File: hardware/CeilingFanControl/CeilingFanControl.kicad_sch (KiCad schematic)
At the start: 28 parts, among them J1 Screw_Terminal_01x02, J2 Conn_01x04, J3 Conn_01x04, J4 Screw_Terminal_01x05, Q1 BTA16-600B, Q2 BTA16-600B, Q3 BTA16-600B, U1 4N25, U2 PIC16F628A-IP, U3 MOC3020M, U4 MOC3020M, U5 MOC3020M, Y1 Crystal

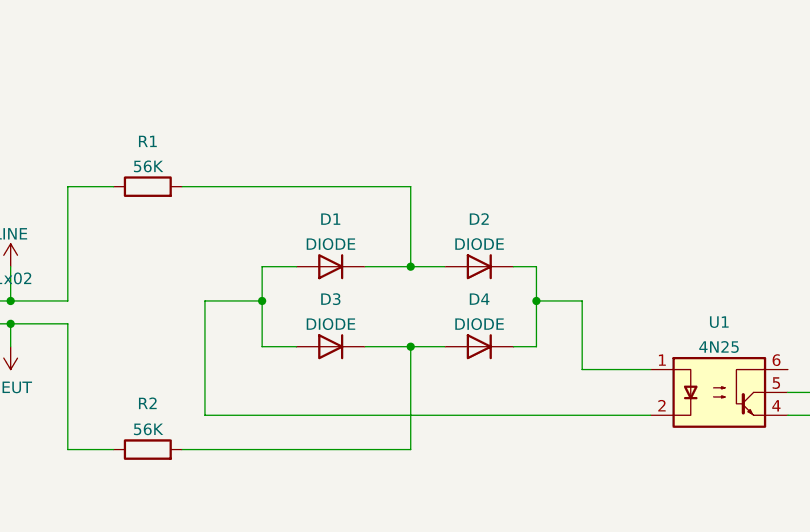
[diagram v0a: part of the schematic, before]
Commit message: Commit befora creating tag
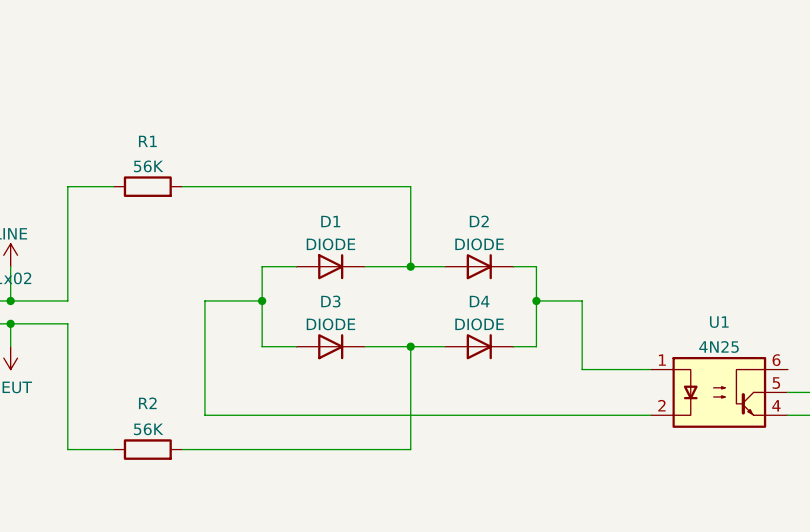
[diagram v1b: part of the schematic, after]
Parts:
- D1, D2, D3, D4: symbol Simulation_SPICE:DIODE -> Diode:1N4001
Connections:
- new net: D2.1 (K), D4.1 (K), U1.1
- new net: D1.1 (K), D2.2 (A), R1.2
- new net: D1.2 (A), D3.2 (A), U1.2
- new net: D3.1 (K), D4.2 (A), R2.2
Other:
- moved on the sheet: D2, D3, D4
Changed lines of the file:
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@@
     (pin "2")
   )
-  (symbol (lib_id "Simulation_SPICE:DIODE") (at 96.52 163.83 0) (mirror x) (unit 1)
-    (in_bom yes) (on_board yes) (fields_autoplaced)
-    (property "Reference" "D2" (id 0) (at 96.52 158.5935 0))
-    (property "Value" "DIODE" (id 1) (at 96.52 161.3686 0))
-    (property "Footprint" "Diode_THT:D_A-405_P7.62mm_Horizontal" (id 2) (at 96.52 163.83 0)
-      (effects (font (size 1.27 1.27)) hide)
-    )
-    (property "Datasheet" "~" (id 3) (at 96.52 163.83 0)
+  (symbol (lib_id "Diode:1N4001") (at 96.52 163.83 180) (unit 1)
+    (in_bom yes) (on_board yes) (fields_autoplaced)
+    (property "Reference" "D2" (id 0) (at 96.52 158.8602 0))
+    (property "Value" "DIODE" (id 1) (at 96.52 161.3971 0))
+    (property "Footprint" "Diode_THT:D_A-405_P7.62mm_Horizontal" (id 2) (at 96.52 159.385 0)
+      (effects (font (size 1.27 1.27)) hide)
+    )
+    (property "Datasheet" "http://www.vishay.com/docs/88503/1n4001.pdf" (id 3) (at 96.52 163.83 0)
       (effects (font (size 1.27 1.27)) hide)
     )
@@
     (pin "1")
   )
-  (symbol (lib_id "Simulation_SPICE:DIODE") (at 80.01 172.72 0) (mirror x) (unit 1)
-    (in_bom yes) (on_board yes) (fields_autoplaced)
-    (property "Reference" "D3" (id 0) (at 80.01 167.4835 0))
-    (property "Value" "DIODE" (id 1) (at 80.01 170.2586 0))
-    (property "Footprint" "Diode_THT:D_A-405_P7.62mm_Horizontal" (id 2) (at 80.01 172.72 0)
-      (effects (font (size 1.27 1.27)) hide)
-    )
-    (property "Datasheet" "~" (id 3) (at 80.01 172.72 0)
+  (symbol (lib_id "Diode:1N4001") (at 80.01 172.72 180) (unit 1)
+    (in_bom yes) (on_board yes) (fields_autoplaced)
+    (property "Reference" "D3" (id 0) (at 80.01 167.7502 0))
+    (property "Value" "DIODE" (id 1) (at 80.01 170.2871 0))
+    (property "Footprint" "Diode_THT:D_A-405_P7.62mm_Horizontal" (id 2) (at 80.01 168.275 0)
+      (effects (font (size 1.27 1.27)) hide)
+    )
+    (property "Datasheet" "http://www.vishay.com/docs/88503/1n4001.pdf" (id 3) (at 80.01 172.72 0)
       (effects (font (size 1.27 1.27)) hide)
     )
@@
     (pin "1")
   )
-  (symbol (lib_id "Simulation_SPICE:DIODE") (at 96.52 172.72 0) (mirror x) (unit 1)
-    (in_bom yes) (on_board yes) (fields_autoplaced)
-    (property "Reference" "D4" (id 0) (at 96.52 167.4835 0))
-    (property "Value" "DIODE" (id 1) (at 96.52 170.2586 0))
-    (property "Footprint" "Diode_THT:D_A-405_P7.62mm_Horizontal" (id 2) (at 96.52 172.72 0)
-      (effects (font (size 1.27 1.27)) hide)
-    )
-    (property "Datasheet" "~" (id 3) (at 96.52 172.72 0)
+  (symbol (lib_id "Diode:1N4001") (at 96.52 172.72 180) (unit 1)
+    (in_bom yes) (on_board yes) (fields_autoplaced)
+    (property "Reference" "D4" (id 0) (at 96.52 167.7502 0))
+    (property "Value" "DIODE" (id 1) (at 96.52 170.2871 0))
+    (property "Footprint" "Diode_THT:D_A-405_P7.62mm_Horizontal" (id 2) (at 96.52 168.275 0)
+      (effects (font (size 1.27 1.27)) hide)
+    )
+    (property "Datasheet" "http://www.vishay.com/docs/88503/1n4001.pdf" (id 3) (at 96.52 172.72 0)
       (effects (font (size 1.27 1.27)) hide)
     )
@@
     (pin "2")
   )
-  (symbol (lib_id "Simulation_SPICE:DIODE") (at 80.01 163.83 0) (unit 1)
-    (in_bom yes) (on_board yes) (fields_autoplaced)
-    (property "Reference" "D1" (id 0) (at 80.01 158.5935 0))
-    (property "Value" "DIODE" (id 1) (at 80.01 161.3686 0))
-    (property "Footprint" "Diode_THT:D_A-405_P7.62mm_Horizontal" (id 2) (at 80.01 163.83 0)
-      (effects (font (size 1.27 1.27)) hide)
-    )
-    (property "Datasheet" "~" (id 3) (at 80.01 163.83 0)
-      (effects (font (size 1.27 1.27)) hide)
-    )
+  (symbol (lib_id "Diode:1N4001") (at 80.01 163.83 0) (mirror y) (unit 1)
+    (in_bom yes) (on_board yes) (fields_autoplaced)
+    (property "Reference" "D1" (id 0) (at 80.01 158.8602 0))
+    (property "Value" "DIODE" (id 1) (at 80.01 161.3971 0))
+    (property "Footprint" "Diode_THT:D_A-405_P7.62mm_Horizontal" (id 2) (at 80.01 168.275 0)
+      (effects (font (size 1.27 1.27)) hide)
+    )
+    (property "Datasheet" "http://www.vishay.com/docs/88503/1n4001.pdf" (id 3) (at 80.01 163.83 0)
+      (effects (font (size 1.27 1.27)) hide)
+    )
